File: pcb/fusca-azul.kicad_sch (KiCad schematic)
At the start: 0 parts

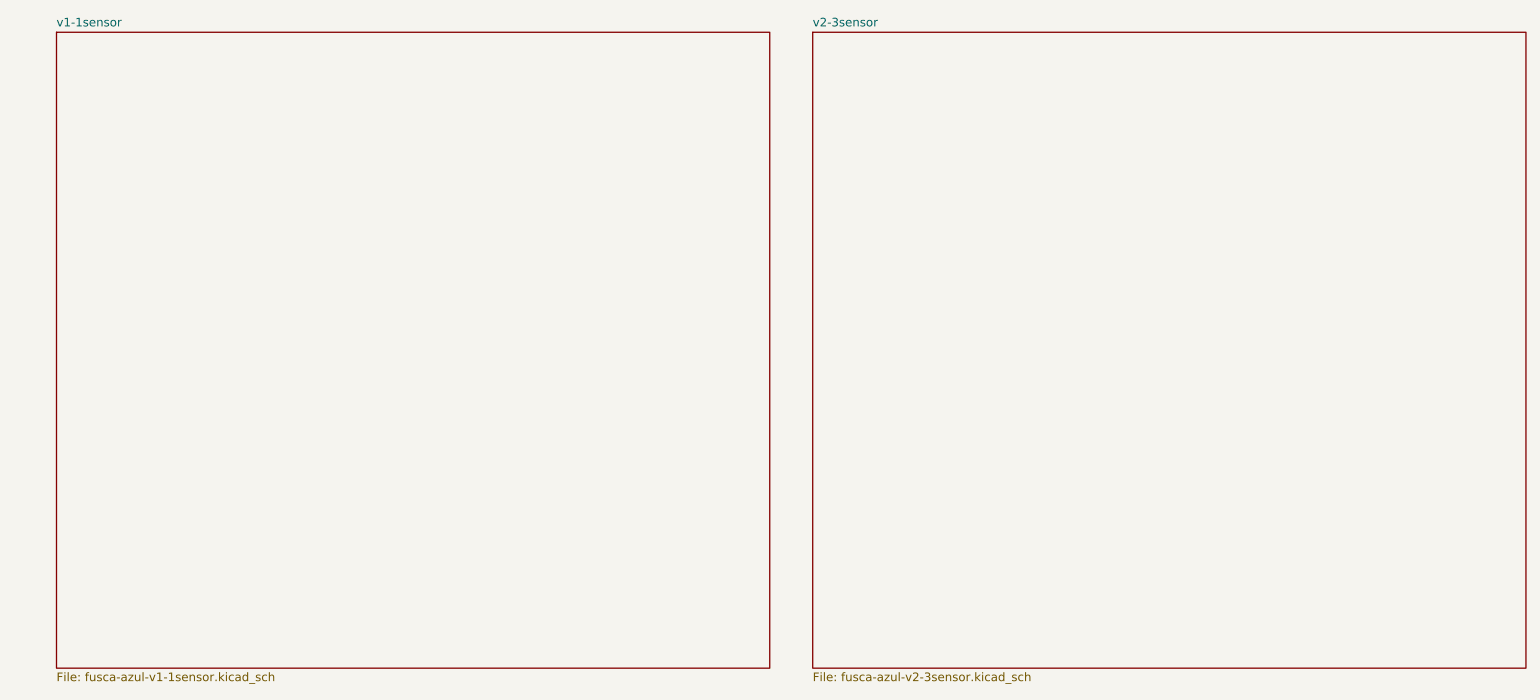
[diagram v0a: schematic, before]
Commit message: feat: atualiza a pcb, mas falta corrigir tamanho e organização
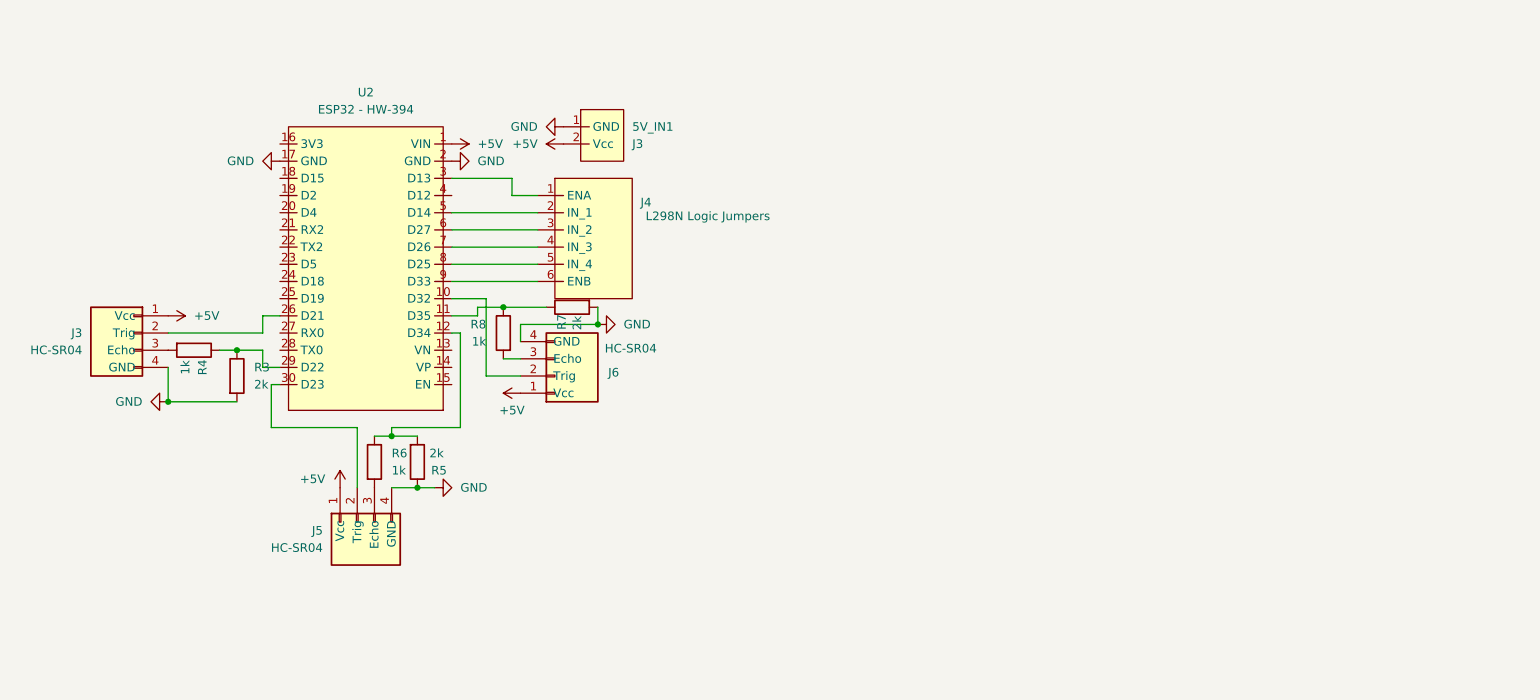
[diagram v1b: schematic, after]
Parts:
- added 5V_IN1: J3, TerminalBlock_Phoenix:TerminalBlock_Phoenix_MKDS-1,5-2-5.08_1x02_P5.08mm_Horizontal, symbol fusca-azul:5V_IN
- added J3, J5, J6: HC-SR04, Connector_PinSocket_2.54mm:PinSocket_1x04_P2.54mm_Vertical, symbol fusca-azul:HC-SR04
- added J4: L298N Logic Jumpers, Connector_PinSocket_2.54mm:PinSocket_1x06_P2.54mm_Vertical, symbol fusca-azul:L298N - Logic Jumpers
- added R3, R5, R7: 2k, Resistor_THT:R_Axial_DIN0207_L6.3mm_D2.5mm_P2.54mm_Vertical, symbol Device:R
- added R4, R6, R8: 1k, Resistor_THT:R_Axial_DIN0207_L6.3mm_D2.5mm_P2.54mm_Vertical, symbol Device:R
- added U2: ESP32 - HW-394, fusca-azul:ESP32-HW-394, symbol fusca-azul:ESP32_-_HW_394
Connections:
- new net: R3.1, R4.1, U2.29 (D22)
- new net: J5.2 (Trig), U2.30 (D23)
- new net: J5.3 (Echo), R6.2
- new net: J4.1 (ENA), U2.3 (D13)
- new net: J4.2 (IN_1), U2.5 (D14)
- new net: J4.3 (IN_2), U2.6 (D27)
- new net: J4.4 (IN_3), U2.7 (D26)
- new net: J4.5 (IN_4), U2.8 (D25)
- new net: J4.6 (ENB), U2.9 (D33)
- new net: R5.2, R6.1, U2.12 (D34)
- new net: J6.2 (Trig), U2.10 (D32)
- new net: J6.3 (Echo), R8.2
- new net: R7.1, R8.1, U2.11 (D35)
- new net: J3.3 (Echo), R4.2
- new net: J3.2 (Trig), U2.26 (D21)
- new net +5V: 5V_IN1.2 (Vcc), J3.1 (Vcc), J5.1 (Vcc), J6.1 (Vcc), U2.1 (VIN)
- new net GND: 5V_IN1.1 (GND), J3.4 (GND), J5.4 (GND), J6.4 (GND), R3.2, R5.1, R7.2, U2.17 (GND), U2.2 (GND)
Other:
- removed sheet v1-1sensor
- removed sheet v2-3sensor

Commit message: feat: finaliza pcb
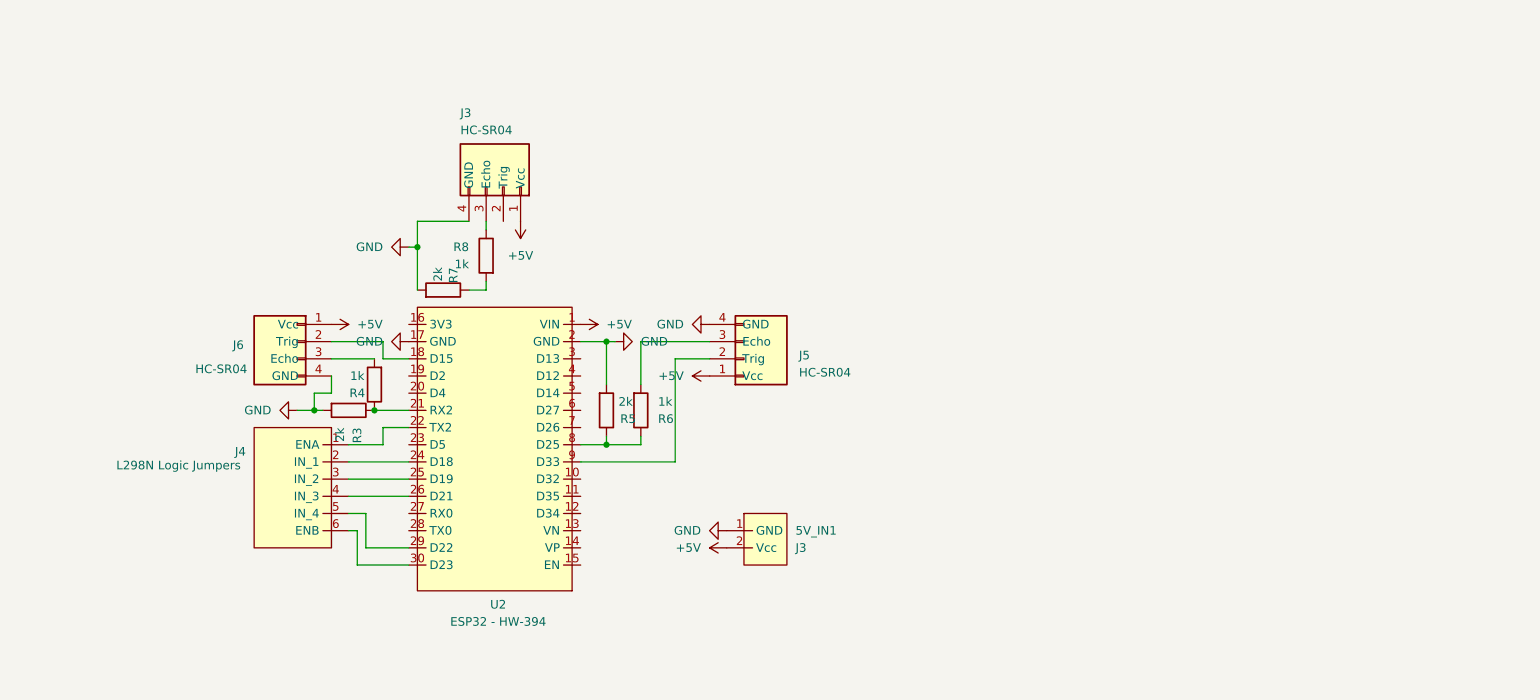
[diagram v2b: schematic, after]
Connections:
- net GND: now also R5.2; no longer R5.1
- net at R3.1, R4.1: now also U2.21 (RX2); no longer U2.29 (D22)
- net at J5.2 (Trig): now also U2.9 (D33); no longer U2.30 (D23)
- net at J4.1 (ENA): now also U2.22 (TX2); no longer U2.3 (D13)
- net at J4.2 (IN_1): now also U2.24 (D18); no longer U2.5 (D14)
- net at J4.3 (IN_2): now also U2.25 (D19); no longer U2.6 (D27)
- net at J4.4 (IN_3): now also U2.26 (D21); no longer U2.7 (D26)
- net at U2.8 (D25): now also R5.1, R6.1; no longer J4.5 (IN_4)
- net at J4.6 (ENB): now also U2.30 (D23); no longer U2.9 (D33)
- net at J6.2 (Trig): now also U2.18 (D15); no longer U2.10 (D32)
- net at J6.3 (Echo): now also R4.2; no longer R8.2
- net at J3.3 (Echo): now also R8.1; no longer R4.2
- net at J3.2 (Trig): no longer U2.26 (D21)
- new net: J4.5 (IN_4), U2.29 (D22)
- new net: R7.1, R8.2
- now unconnected: U2.11 (D35), U2.12 (D34)
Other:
- moved on the sheet: 5V_IN1, J3, J4, J5, U2

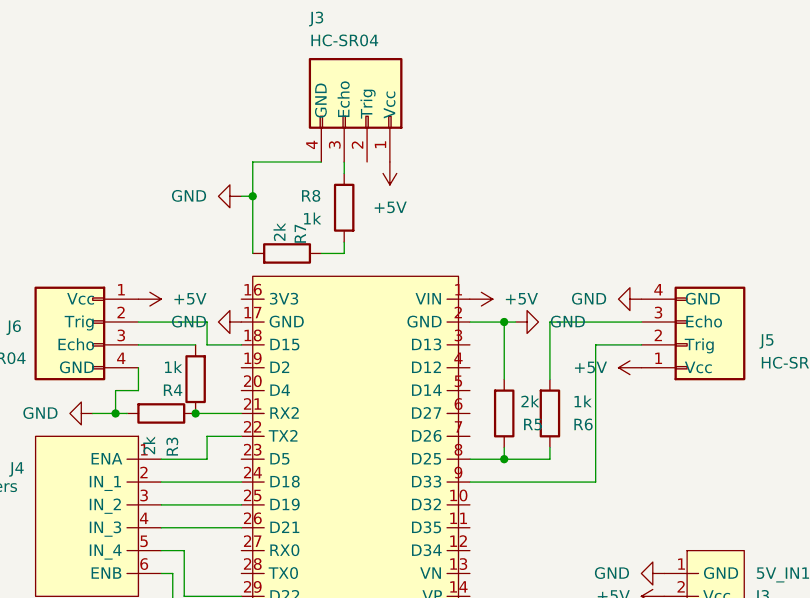
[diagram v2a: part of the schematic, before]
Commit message: fix: corrige ligacao na placa
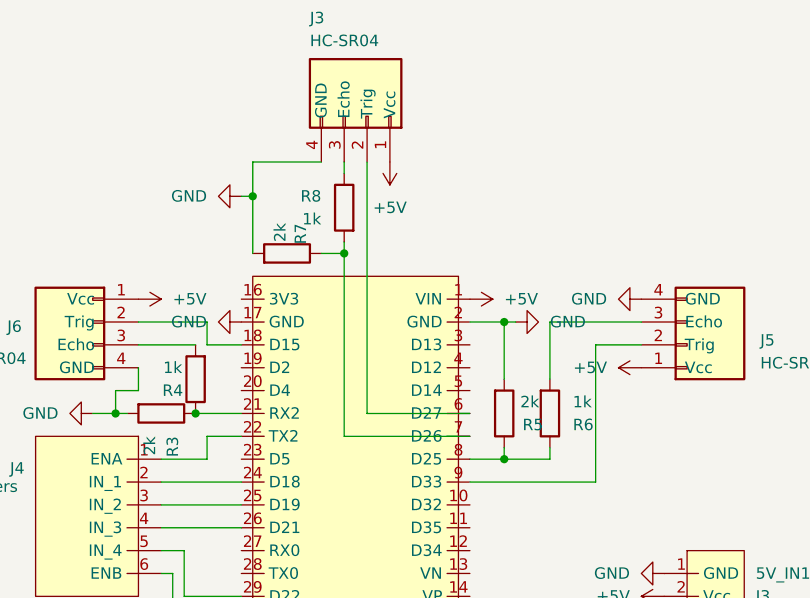
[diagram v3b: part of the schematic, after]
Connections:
- net at R7.1, R8.2: now also U2.7 (D26)
- net at J3.2 (Trig): now also U2.6 (D27)
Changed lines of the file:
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@@
 	(paper "A4")
 	(junction
+		(at 86.36 57.15)
+		(diameter 0)
+		(color 0 0 0 0)
+	)
+	(junction
 		(at 104.14 64.77)
 		(diameter 0)
@@
 	(wire
 		(pts
+			(xy 100.33 77.47) (xy 86.36 77.47)
+		)
+		(stroke
+			(width 0)
+			(type default)
+		)
+	)
+	(wire
+		(pts
 			(xy 74.93 97.79) (xy 67.31 97.79)
 		)
@@
 	(wire
 		(pts
+			(xy 88.9 74.93) (xy 100.33 74.93)
+		)
+		(stroke
+			(width 0)
+			(type default)
+		)
+	)
+	(wire
+		(pts
 			(xy 66.04 90.17) (xy 68.58 90.17)
 		)
@@
 	(wire
 		(pts
+			(xy 88.9 46.99) (xy 88.9 74.93)
+		)
+		(stroke
+			(width 0)
+			(type default)
+		)
+	)
+	(wire
+		(pts
 			(xy 104.14 71.12) (xy 104.14 64.77)
 		)
@@
 		)
 		(stroke
+			(width 0)
+			(type default)
+		)
+	)
+	(wire
+		(pts
+			(xy 86.36 77.47) (xy 86.36 57.15)
+		)
+		(stroke

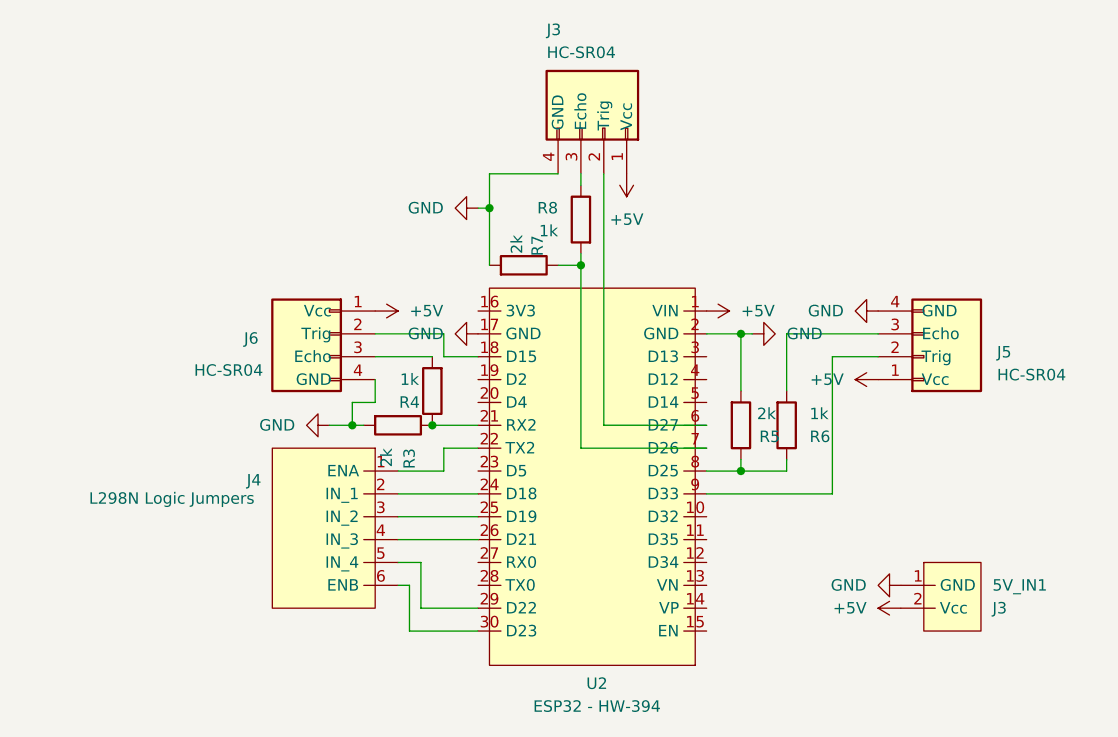
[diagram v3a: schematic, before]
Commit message: finaliza pcb
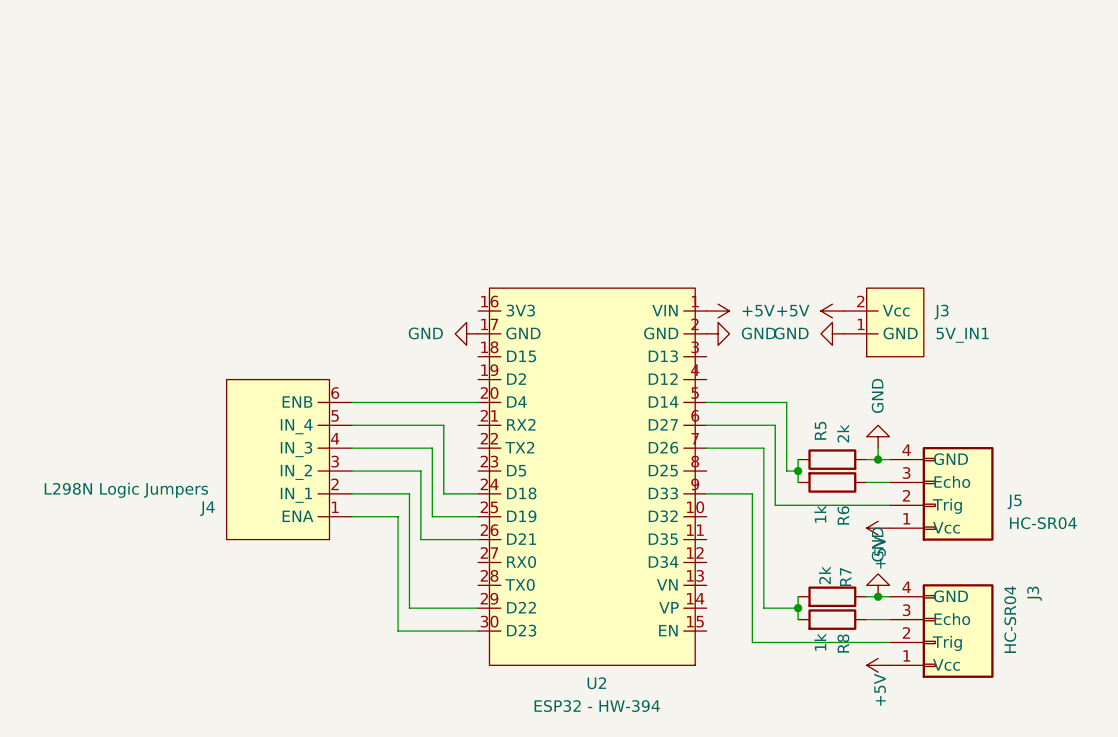
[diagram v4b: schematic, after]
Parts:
- removed J6: HC-SR04, Connector_PinSocket_2.54mm:PinSocket_1x04_P2.54mm_Vertical, symbol fusca-azul:HC-SR04
- removed R3: 2k, Resistor_THT:R_Axial_DIN0207_L6.3mm_D2.5mm_P2.54mm_Vertical, symbol Device:R
- removed R4: 1k, Resistor_THT:R_Axial_DIN0207_L6.3mm_D2.5mm_P2.54mm_Vertical, symbol Device:R
- R5, R6, R7, R8: footprint Resistor_THT:R_Axial_DIN0207_L6.3mm_D2.5mm_P2.54mm_Vertical -> Resistor_THT:R_Axial_DIN0207_L6.3mm_D2.5mm_P5.08mm_Vertical
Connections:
- net GND: now also R7.1; no longer R7.2
- net at J5.3 (Echo): now also R6.1; no longer R6.2
- net at U2.9 (D33): now also J3.2 (Trig); no longer J5.2 (Trig)
- net at J4.1 (ENA): now also U2.30 (D23); no longer U2.22 (TX2)
- net at J4.2 (IN_1): now also U2.29 (D22); no longer U2.24 (D18)
- net at J4.3 (IN_2): now also U2.26 (D21); no longer U2.25 (D19)
- net at J4.4 (IN_3): now also U2.25 (D19); no longer U2.26 (D21)
- net at J4.5 (IN_4): now also U2.24 (D18); no longer U2.29 (D22)
- net at J4.6 (ENB): now also U2.20 (D4); no longer U2.30 (D23)
- net at R8.2, U2.7 (D26): now also R7.2; no longer R7.1
- net at U2.6 (D27): now also J5.2 (Trig); no longer J3.2 (Trig)
- net at U2.5 (D14): now also R5.1, R6.2
- now unconnected: U2.8 (D25)
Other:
- moved on the sheet: 5V_IN1, J4, R5, R6, R7, R8
